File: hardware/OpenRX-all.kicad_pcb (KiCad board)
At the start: 6 copper layers, 86.5 x 17.6 mm, 343 parts, among them J1 Conn_Coaxial_Small, J2 Conn_Coaxial_Small, J3 Conn_Coaxial_Small, J4 Conn_Coaxial_Small, J5 Conn_Coaxial, J6 Conn_Coaxial_Small, T1 0900PC16J0042001E, T2 0900PC16J0042001E, T3 0900PC16J0042001E, T4 0900PC16J0042001E, T5 0900PC16J0042001E, U1 ESP32-C3, U10 ESP32-C3, U11 TLV75533PDQNR, U12 LR1121IMLTRT, U13 RFX2401C, U14 SKY13373-460LF, U15 LR1121IMLTRT, U16 RFX2401C, U17 SKY13373-460LF, U18 TS2306A 240GF MSM 9_C2976675, U19 ESP32-C3, U2 TLV75533PDQNR, U20 TLV75533PDQNR, U21 SX1281IMLTRT, U22 ESP32-C3, U23 TLV75533PDQNR, U24 SX1281IMLTRT, U25 ESP32-C3, U26 TLV75533PDQNR, U27 LR1121IMLTRT, U28 RFX2401C, U29 SKY13373-460LF, U3 LR1121IMLTRT, U4 RFX2401C, U5 SKY13373-460LF, U6 LR1121IMLTRT, U7 RFX2401C, U8 SKY13373-460LF, U9 TS2306A 240GF MSM 9_C2976675, X1 CJ17-400001010B20, X2 CJ17-400001010B20, X3 CJ17-400001010B20, X4 CJ17-400001010B20, X5 CJ17-400001010B20

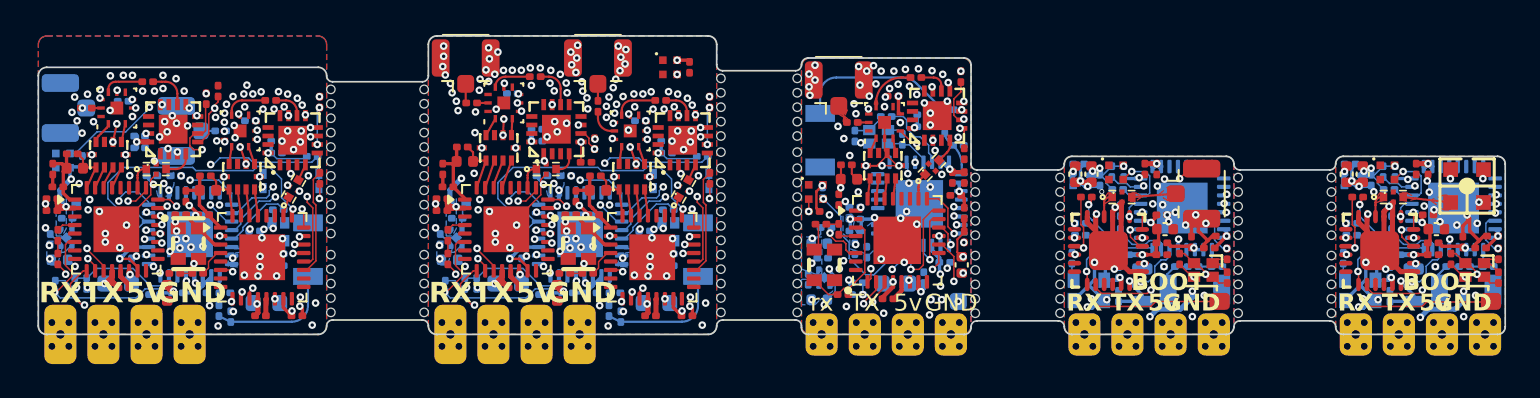
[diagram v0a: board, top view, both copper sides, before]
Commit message: updated HW files as ordered
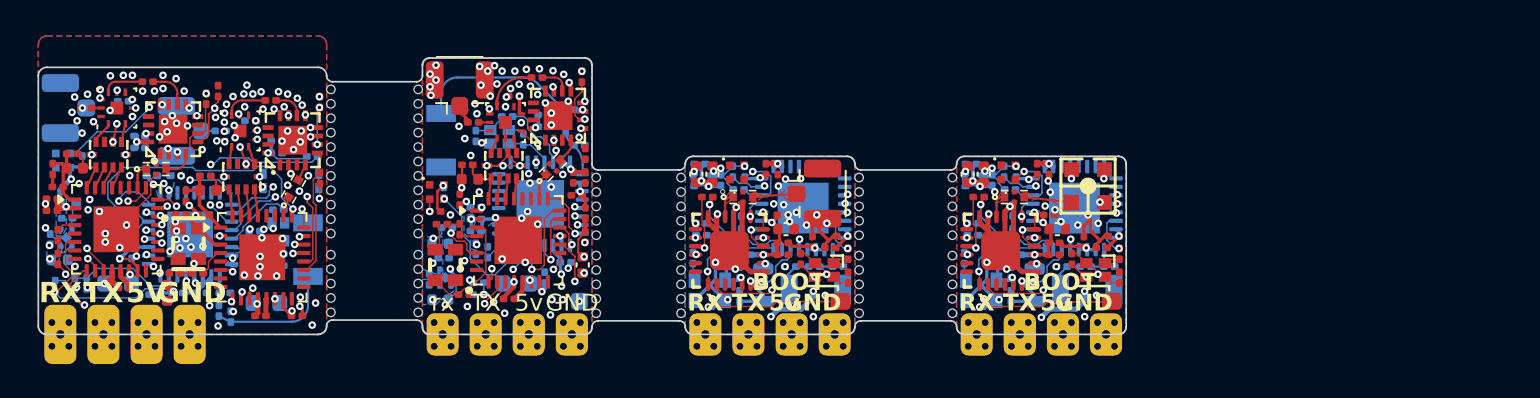
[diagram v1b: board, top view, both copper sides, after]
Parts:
- removed AE2: 2450AT18A100E, OpenRX-Shared:ANT-SMD_L3.2-W1.6
- removed C32, C46: 15pF, Capacitor_SMD:C_0201_0603Metric
- removed C45, C66, C67, C81, C84, C86: 47p, Capacitor_SMD:C_0201_0603Metric
- removed C47, C53, C60, C68, C70, C71, C74, C83: 1uF, Capacitor_SMD:C_0201_0603Metric
- removed C48, C49, C52, C55, C56, C57, C59, C77, C79: 100nF, Capacitor_SMD:C_0201_0603Metric
- removed C50, C76: 10pF, Capacitor_SMD:C_0201_0603Metric
- removed C51, C54, C61: 10uF, Capacitor_SMD:C_0402_1005Metric
- removed C58, C78: 47pF, Capacitor_SMD:C_0201_0603Metric
- removed C62, C75: 2.2nF, Capacitor_SMD:C_0201_0603Metric
- removed C63, C80: 470nF, Capacitor_SMD:C_0201_0603Metric
- removed C64, C82: 220pF, Capacitor_SMD:C_0201_0603Metric
- removed C65, C85: 1n, Capacitor_SMD:C_0201_0603Metric
- removed C69: 10nF, Capacitor_SMD:C_0201_0603Metric
- removed C72, C73: 1.2pF, Capacitor_SMD:C_0201_0603Metric
- removed D2: XL-1010RGBC-WS2812B, OpenRX-Shared:LED-SMD_4P-L1.0-W1.0-TL_XL-1010RGBC-WS2812B
- removed FL3, FL4: 2450FM07D0034T, OpenRX-Shared:FILTER-SMD_4P-L1.0-W0.5-L
- removed J3, J4: Conn_Coaxial_Small, Connector_Coaxial:U.FL_Hirose_U.FL-R-SMT-1_Vertical
- removed L10: 2.0nH, Inductor_SMD:L_0201_0603Metric
- removed L11: 2.5nH, Inductor_SMD:L_0201_0603Metric
- removed L12, L14: 47nH, Inductor_SMD:L_0402_1005Metric
- removed L13, L8: 10uH, Inductor_SMD:L_0603_1608Metric
- removed L9: 24nH, Inductor_SMD:L_0201_0603Metric
- removed OSC2: OW7EL89CENUYO3YLC-32M, OpenRX-Shared:OSC-SMD_4P-L2.0-W1.6-BL_TXC_7Z
- removed R13, R22: 200, Resistor_SMD:R_0201_0603Metric
- removed R14, R15, R16, R17: 10k, Resistor_SMD:R_0201_0603Metric
- removed R18, R21: 220, Resistor_SMD:R_0201_0603Metric
- removed R19, R20, R23, R24: 100k, Resistor_SMD:R_0201_0603Metric
- removed the REF** at (140.2, 111.5)
- removed the REF** at (122.8, 114.0)
- removed the REF** at (140.2, 106.2)
- removed the REF** at (144.8, 111.5)
- removed the REF** at (144.8, 103.6)
- removed the REF** at (122.8, 106.8)
- removed the REF** at (140.2, 103.6)
- removed the REF** at (144.8, 106.2)
- removed T3, T4: 0900PC16J0042001E, OpenRX-Shared:FILTER-SMD_10P-L2.0-W1.6-BL
- removed TP5: RX, OpenRX-Shared:SolderPad_1.2x2.0mm
- removed TP6: TX, OpenRX-Shared:SolderPad_1.2x2.0mm
- removed TP7: 5V, OpenRX-Shared:SolderPad_1.2x2.0mm
- removed TP8: GND, OpenRX-Shared:SolderPad_1.2x2.0mm
- removed U10: ESP32-C3, Package_DFN_QFN:QFN-32-1EP_5x5mm_P0.5mm_EP3.7x3.7mm
- removed U11: TLV75533PDQNR, OpenRX-Shared:X2SON-4_L1.0-W1.0-P0.65-TL-EP
- removed U12, U15: LR1121IMLTRT, Package_DFN_QFN:QFN-32-1EP_5x5mm_P0.5mm_EP3.7x3.7mm
- removed U13, U16: RFX2401C, OpenRX-Shared:QFN-16_L3.0-W3.0-P0.50-BL-EP1.7
- removed U14, U17: SKY13373-460LF, OpenRX-Shared:QFN-12_EP_2x2_Pitch0.5mm
- removed U18: TS2306A 240GF MSM 9_C2976675, OpenRX-Shared:SW-SMD_4P-L3.0-W2.0-P0.85-LS3.5
- removed X2: CJ17-400001010B20, OpenRX-Shared:CRYSTAL-SMD_4P-L1.6-W1.2-BL
- added REF**: BreakLine_11h_D0.5mm_P0.85mm, Panelization:BreakLine_11h_D0.5mm_P0.85mm, F.Cu at (122.4, 106.8)
- added REF**: BreakLine_5h_D0.5mm_P0.85mm, Panelization:BreakLine_5h_D0.5mm_P0.85mm, F.Cu at (122.4, 114.0)
- moved C111 22.4 mm to (141.4, 109.7)
- moved C113 22.4 mm to (160.9, 112.5)
- moved C114 22.4 mm to (162.7, 111.9)
- moved C136 22.4 mm to (157.4, 109.7)
- moved C88 22.4 mm to (144.9, 112.5)
- moved C89 22.4 mm to (146.7, 111.9)
- moved D3 22.4 mm to (141.2, 107.5)
- moved D4 22.4 mm to (157.2, 107.5)
- moved L23 22.4 mm to (128.2, 114.0)
- moved R25 22.4 mm to (139.4, 108.9)
- moved R27 22.4 mm to (140.9, 107.4)
- moved R28 22.4 mm to (141.4, 111.1)
- moved R29 22.4 mm to (155.4, 108.9)
- moved R31 22.4 mm to (156.9, 107.4)
- moved R32 22.4 mm to (157.4, 111.1)
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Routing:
- net Net-(U1-U0TXD): track 102.5 -> 69.6 mm, vias 5 -> 4
- net +3V3: track 115.0 -> 87.5 mm, vias 73 -> 54
- net Net-(U1-U0RXD): track 83.6 -> 61.2 mm, vias 7 -> 5
- net GND: track 119.1 -> 97.9 mm, vias 375 -> 234
- net /ESP32-C3/DIO1_B: track 39.3 -> 19.6 mm, vias 4 -> 2
- net /ESP32-C3/BUSY_B: track 37.8 -> 18.9 mm, vias 2 -> 1
- net /ESP32-C3/RST_B: track 32.9 -> 16.4 mm, vias 4 -> 2
- net /LR1121_A/TXEN24: track 35.2 -> 19.8 mm, vias 4 -> 2
- net /ESP32-C3/MOSI: track 30.0 -> 15.0 mm, vias 6 -> 3
- net /LR1121_B/CTRL2: track 29.8 -> 14.9 mm, vias 4 -> 2
- net /ESP32-C3/BOOT: track 29.6 -> 14.8 mm, vias 4 -> 2
- net /LR1121_A/CTRL2: track 28.1 -> 14.4 mm, vias 4 -> 2
- net /ESP32-C3/MISO: track 26.9 -> 13.4 mm, vias 6 -> 3
- net /LR1121_A/CTRL1: track 25.8 -> 12.8 mm, vias 4 -> 2
- net /ESP32-C3/SCK: track 25.8 -> 12.9 mm, vias 6 -> 3
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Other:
- board size 86.5 x 17.6 mm -> 64.2 x 16.3 mm
